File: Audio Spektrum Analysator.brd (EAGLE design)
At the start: 144.8 x 98.7 mm, 159 parts, among them IC1 LM324N, IC10 LM3914N, IC11 LM3914N, IC12 LM3914N, IC13 LM3914N, IC2 LM324N, IC3 LM324N, IC4 LM3914N, IC5 LM3914N, IC6 LM3914N, IC7 LM3914N, IC8 LM3914N, IC9 LM3914N, J2 DCJ0202, M1 ELECTRET_MICROPHON-F6050AP

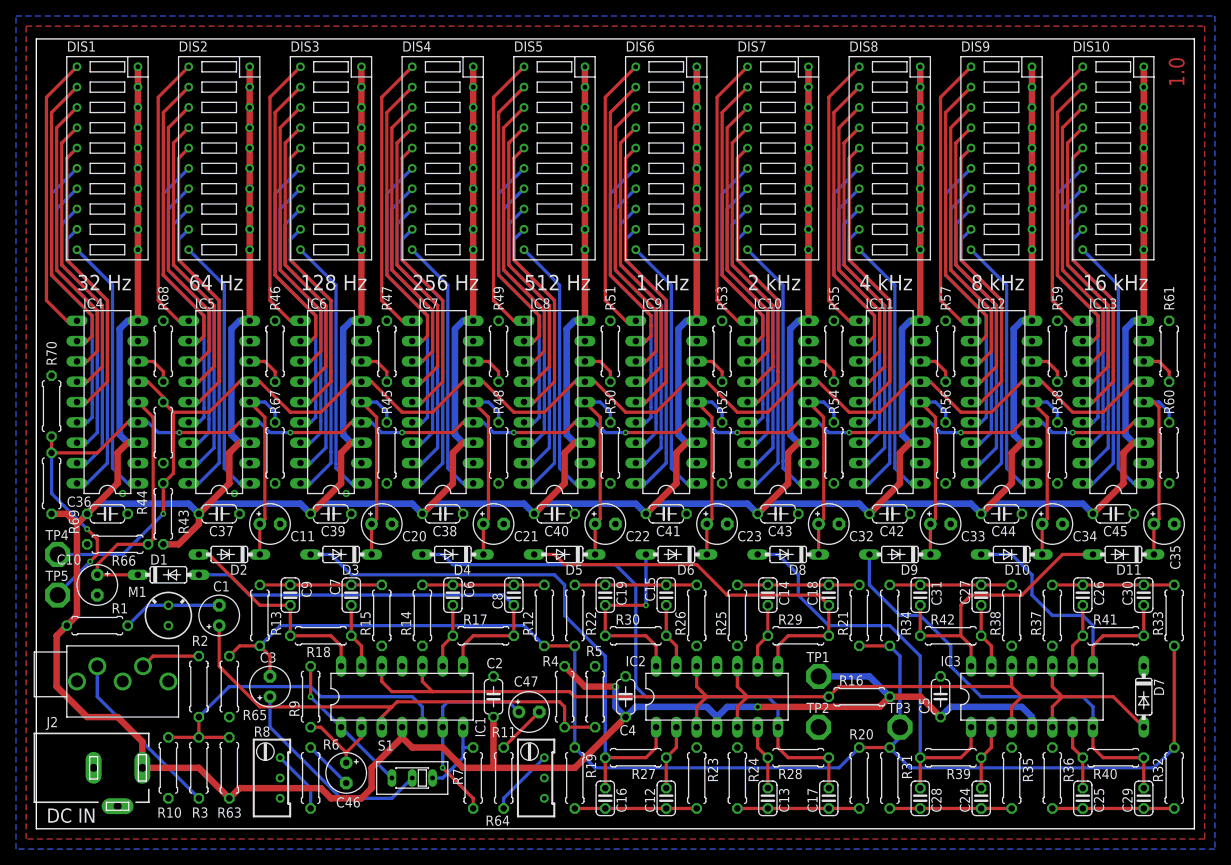
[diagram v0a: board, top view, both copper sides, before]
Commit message: Ich habe fertig V1.0
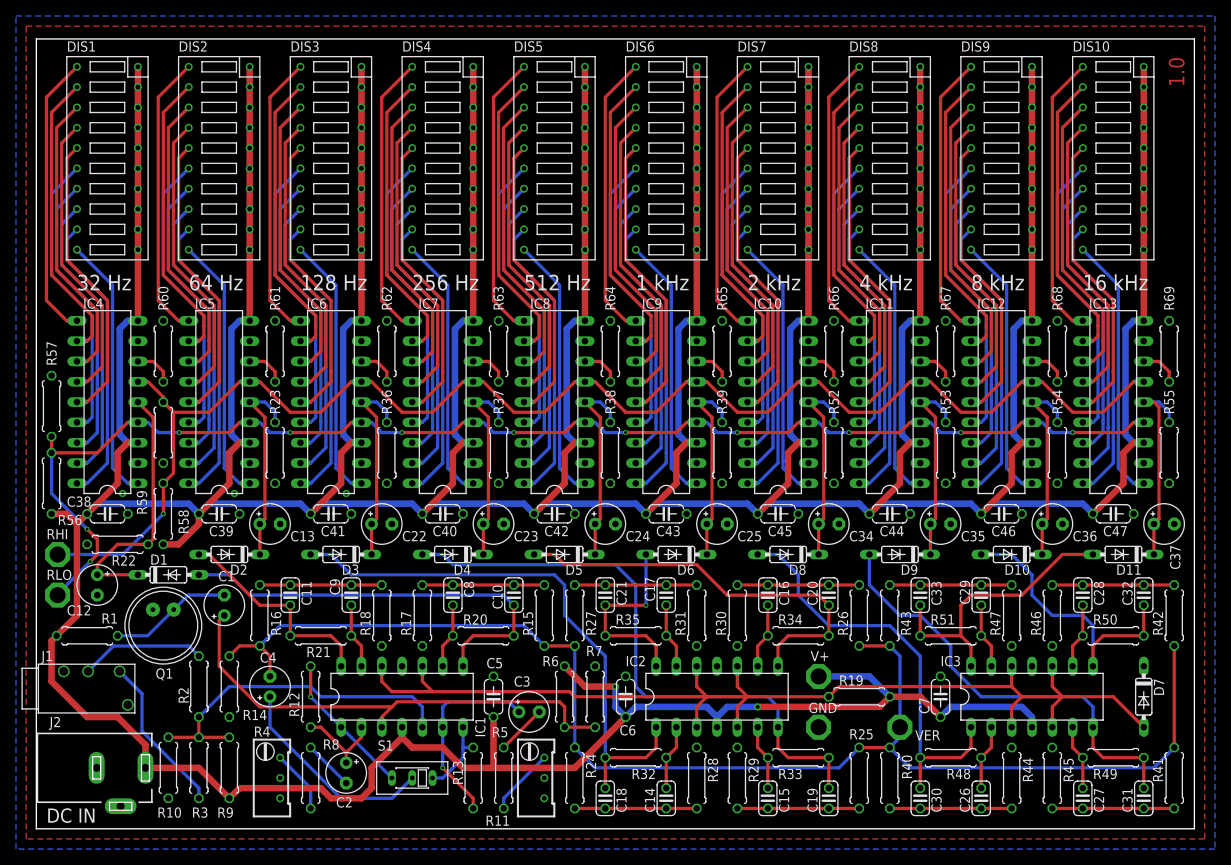
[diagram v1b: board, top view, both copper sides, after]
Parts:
- removed M1: ELECTRET_MICROPHON-F6050AP, microphon:F6050AP
- removed R70: 1k, resistor:0207/7
- added Q1: (no value), adafruit:9.7ELECTRET
- added R62: 1k2, resistor:0207/7
- C10: value 1u -> 22n; device resistor:E2,5-5 -> resistor:C025-024X044
- C11: value 1u -> 10n; device resistor:E2,5-5 -> resistor:C025-024X044
- C12: value 4n7 -> 1u; device resistor:C025-024X044 -> resistor:E2,5-5
- C13: value 2n2 -> 1u; device resistor:C025-024X044 -> resistor:E2,5-5
- C14, C18: value 1n2 -> 4n7
- C15, C19: value 620p -> 2n2
- C16: value 4n7 -> 1n2
- C17: value 2n2 -> 620p
- C2, C4: value 100n -> 2u2; device resistor:C050-024X044 -> resistor:E2,5-5
- C20: value 1u -> 1n2; device resistor:E2,5-5 -> resistor:C025-024X044
- C21: value 1u -> 620p; device resistor:E2,5-5 -> resistor:C025-024X044
- C24: value 330p -> 1u; device resistor:C025-024X044 -> resistor:E2,5-5
- C25: value 160p -> 1u; device resistor:C025-024X044 -> resistor:E2,5-5
- C26, C30: value 82p -> 330p
- C27, C31: value 39p -> 160p
- C28: value 330p -> 82p
- C29: value 160p -> 39p
- C32: value 1u -> 82p; device resistor:E2,5-5 -> resistor:C025-024X044
- C33: value 1u -> 39p; device resistor:E2,5-5 -> resistor:C025-024X044
- C36, C37: value 100n -> 1u; device resistor:C050-024X044 -> resistor:E2,5-5
- C46, C47: value 2u2 -> 100n; device resistor:E2,5-5 -> resistor:C050-024X044
- C6: value 22n -> 100n; device resistor:C025-024X044 -> resistor:C050-024X044
- C7: value 10n -> 100n; device resistor:C025-024X044 -> resistor:C050-024X044
- J1: device Jakobs_LBR:2.5MM-AUX_PC -> Jakobs_LBR:2,5MM-AUX_JACK
- R11: value 50k -> 1k; device resistor:RTRIM64W -> rcl:0207/7
- R12, R22, R23, R36, R37, R38: value 120k -> 100k; device resistor:0207/7 -> rcl:0207/7
- R13: value 120k -> 10k
- R14: value 120k -> 1M; device resistor:0207/7 -> rcl:0207/7
- R16: value 22k -> 120k
- R17, R18, R27, R28, R29, R30, R40, R41, R42: value 1M -> 120k
- R19: value 120k -> 22k
- R20, R21, R32, R33, R34, R35: value 120k -> 1M
- R39: value 1M -> 100k; device resistor:0207/7 -> rcl:0207/7
- R4: value 47k -> 10k; device rcl:0207/7 -> resistor:RTRIM64W
- R43, R44: value 20k -> 120k
- R45: value 100k -> 120k; device rcl:0207/7 -> resistor:0207/7
- R46, R47: value 1k2 -> 120k
- R48, R50: value 100k -> 1M; device rcl:0207/7 -> resistor:0207/7
- R49, R51: value 1k2 -> 1M
- R5: value 47k -> 50k; device rcl:0207/7 -> resistor:RTRIM64W
- R53, R55: value 1k2 -> 100k; device resistor:0207/7 -> rcl:0207/7
- R56: value 100k -> 9k; device rcl:0207/7 -> resistor:0207/7
- R57: value 1k2 -> 1k
- R58: value 100k -> 20k; device rcl:0207/7 -> resistor:0207/7
- R59: value 1k2 -> 20k
- R6: value 10k -> 47k
- R60, R66, R67: value 100k -> 1k2; device rcl:0207/7 -> resistor:0207/7
- R63: value 47k -> 1k2; device rcl:0207/7 -> resistor:0207/7
- R64: value 1k -> 1k2; device rcl:0207/7 -> resistor:0207/7
- R65: value 1M -> 1k2; device rcl:0207/7 -> resistor:0207/7
- R69: value 9k -> 1k2
- R7: value 10k -> 47k; device resistor:0207/7 -> rcl:0207/7
- R8: device resistor:RTRIM64W -> rcl:0207/7
- R9: value 100k -> 47k
- moved R69 140.7 mm to (141.6, 59.7)
- moved R60 126.4 mm to (15.9, 59.7), turned to 270 degrees
- moved C36 118.1 mm to (127.0, 38.1)
- moved C37 118.1 mm to (141.0, 38.1)
- moved R44 114.5 mm to (121.9, 6.35), turned to 270 degrees
- moved R59 112.2 mm to (15.9, 49.5), turned to 90 degrees
- moved R58 112.0 mm to (15.9, 39.4), turned to 270 degrees
- moved R57 112.0 mm to (1.91, 52.8)
- moved R56 111.8 mm to (1.91, 43.2), turned to 270 degrees
- moved R68 111.8 mm to (127.6, 59.7)
- moved R61 111.8 mm to (29.8, 59.7)
- moved R46 102.6 mm to (127.0, 26.7), turned to 90 degrees
- moved R66 92.7 mm to (99.7, 59.7), turned to 270 degrees
- moved R36 92.6 mm to (43.8, 47.0), turned to 90 degrees
- moved R45 92.6 mm to (127.0, 6.35), turned to 270 degrees
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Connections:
- net GND: now also C12.-, C13.-, C24.-, C25.-, C36.-, C37.-, C46.2, C47.2, C6.2, C7.2, J1.4, J2.2, Q1.-, R17.1, R18.1, R22.1, R28.1, R29.1, R30.1, R31.1, R39.1, R4.2, R5.2, R62.1, R63.1, R64.1, R69.1, R7.1; no longer C10.-, C11.-, C2.2, C20.-, C21.-, C32.-, C33.-, C36.2, C37.2, C4.2, M1.1, R11.2, R15.1, R24.1, R25.1, R26.1, R35.1, R48.1, R49.1, R5.1, R50.1, R51.1, R56.1, R58.1, R70.1, R8.2
- net N$1: now also J1.2; no longer J1.4
- net N$10: now also R13.2; no longer R7.2
- net N$108: now also R60.2; no longer R68.2
- net N$12: now also C4.+; no longer C3.+
- net N$125: now also C18.2, R32.2; no longer C16.2, R27.2
- net N$13: now also Q1.+; no longer M1.2
- net N$130: now also C14.2, R32.1; no longer C12.2, R27.1
- net N$133: now also C10.2, R20.2; no longer C8.2, R17.2
- net N$134: now also C8.2, R20.1; no longer C6.2, R17.1
- net N$135: now also C21.2, R35.2; no longer C19.2, R30.2
- net N$136: now also C10.1, R15.2, R17.2; no longer C6.1, R12.2, R14.2
- net N$138: now also C11.2, R21.2; no longer C9.2, R18.2
- net N$139: now also C9.2, R21.1; no longer C7.2, R18.1
- net N$140: now also C14.1, C18.1, R24.2, R28.2; no longer C12.1, C16.1, R19.2, R23.2
- net N$141: now also C11.1, R16.2, R18.2; no longer C7.1, R13.2, R15.2
- net N$144: now also C19.2, R33.2; no longer C17.2, R28.2
- net N$145: now also C15.2, R33.1; no longer C13.2, R28.1
- net N$146: now also C17.2, R35.1; no longer C15.2, R30.1
- net N$147: now also C15.1, C19.1, R25.2, R29.2; no longer C13.1, C17.1, R20.2, R24.2
- net N$149: now also C20.2, R34.2; no longer C18.2, R29.2
- net N$150: now also C16.2, R34.1; no longer C14.2, R29.1
- net N$151: now also C30.2, R48.2; no longer C28.2, R39.2
- net N$152: now also C16.1, C20.1, R26.2, R30.2; no longer C14.1, C18.1, R21.2, R25.2
- net N$154: now also C17.1, C21.1, R27.2, R31.2; no longer C15.1, C19.1, R22.2, R26.2
- net N$156: now also C26.2, R48.1; no longer C24.2, R39.1
- net N$157: now also C26.1, C30.1, R40.2, R44.2; no longer C24.1, C28.1, R31.2, R35.2
- net N$159: now also C31.2, R49.2; no longer C29.2, R40.2
- net N$160: now also C27.2, R49.1; no longer C25.2, R40.1
- net N$161: now also C27.1, C31.1, R41.2, R45.2; no longer C25.1, C29.1, R32.2, R36.2
- net N$163: now also C32.2, R50.2; no longer C30.2, R41.2
- net N$164: now also C28.2, R50.1; no longer C26.2, R41.1
- net N$165: now also C28.1, C32.1, R42.2, R46.2; no longer C26.1, C30.1, R33.2, R37.2
- net N$167: now also C33.2, R51.2; no longer C31.2, R42.2
- net N$168: now also C29.2, R51.1; no longer C27.2, R42.1
- net N$169: now also C29.1, C33.1, R43.2, R47.2; no longer C27.1, C31.1, R34.2, R38.2
- net N$2: now also J1.3; no longer J1.2
- net N$29: now also R62.2; no longer R47.2
- net N$3: now also R9.1; no longer R63.1
- net N$30: now also R61.2; no longer R46.2
- net N$31: now also C2.-, R8.2; no longer C46.-, R6.2
- net N$4: now also R6.1, R7.2; no longer R4.1, R5.2
- net N$42: now also R63.2; no longer R49.2
- net N$43: now also R64.2; no longer R51.2
- net N$44: now also R4.3, R8.1; no longer R6.1, R8.3
- net N$5: now also C2.+, R12.1; no longer C46.+, R9.1
- net N$55: now also R66.2; no longer R55.2
- net N$56: now also R65.2; no longer R53.2
- net N$57: now also C3.+, R13.1; no longer C47.+, R7.1
- net N$6: now also R12.2; no longer R9.2
- net N$68: now also R67.2; no longer R57.2
- net N$69: now also R68.2; no longer R59.2
- net N$70: now also C3.-, R11.2; no longer C47.-, R64.2
- net N$81: now also R69.2; no longer R61.2
- net N$83: now also R11.1, R5.3; no longer R11.3, R64.1
- net OUT1: now also C12.+, R22.2; no longer C10.+, R66.2
- net OUT10: now also C37.+, R55.2; no longer C35.+, R60.2
- net OUT2: now also C13.+, R23.2; no longer C11.+, R67.2
- net OUT3: now also C22.+, R36.2; no longer C20.+, R45.2
- net OUT4: now also C23.+, R37.2; no longer C21.+, R48.2
- net OUT5: now also C24.+, R38.2; no longer C22.+, R50.2
- net OUT6: now also C25.+, R39.2; no longer C23.+, R52.2
- net OUT7: now also C34.+, R52.2; no longer C32.+, R54.2
- net OUT8: now also C35.+, R53.2; no longer C33.+, R56.2
- net OUT9: now also C36.+, R54.2; no longer C34.+, R58.2
- net REF: now also R19.1; no longer R16.1
- net RHI: now also R58.1, R59.2; no longer R43.1, R44.2
- net RLO: now also R56.1, R57.2; no longer R69.1, R70.2
- net V+: now also C46.1, C47.1, C6.1, C7.1, R19.2, R56.2, R58.2, R6.2, R9.2; no longer C2.1, C36.1, C37.1, C4.1, R16.2, R4.2, R43.2, R63.2, R69.2
- net VER: now also C4.-, R14.2, R15.1, R16.1, R24.1, R25.1, R26.1, R27.1, R40.1, R41.1, R42.1, R43.1; no longer C3.-, R12.1, R13.1, R19.1, R20.1, R21.1, R22.1, R31.1, R32.1, R33.1, R34.1, R65.2
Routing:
- net N$1: track 7.51 -> 15.7 mm
- net N$13: track 12.5 -> 15.4 mm
- net N$2: track 21.8 -> 20.0 mm
- net N$4: track 60.3 -> 61.8 mm
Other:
- board text added: "GND"
- board text added: "RHI"
- board text added: "RLO"
- board text added: "V+"
- board text added: "VER"
